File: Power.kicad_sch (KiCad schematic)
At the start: 19 parts, among them U2 sct2620

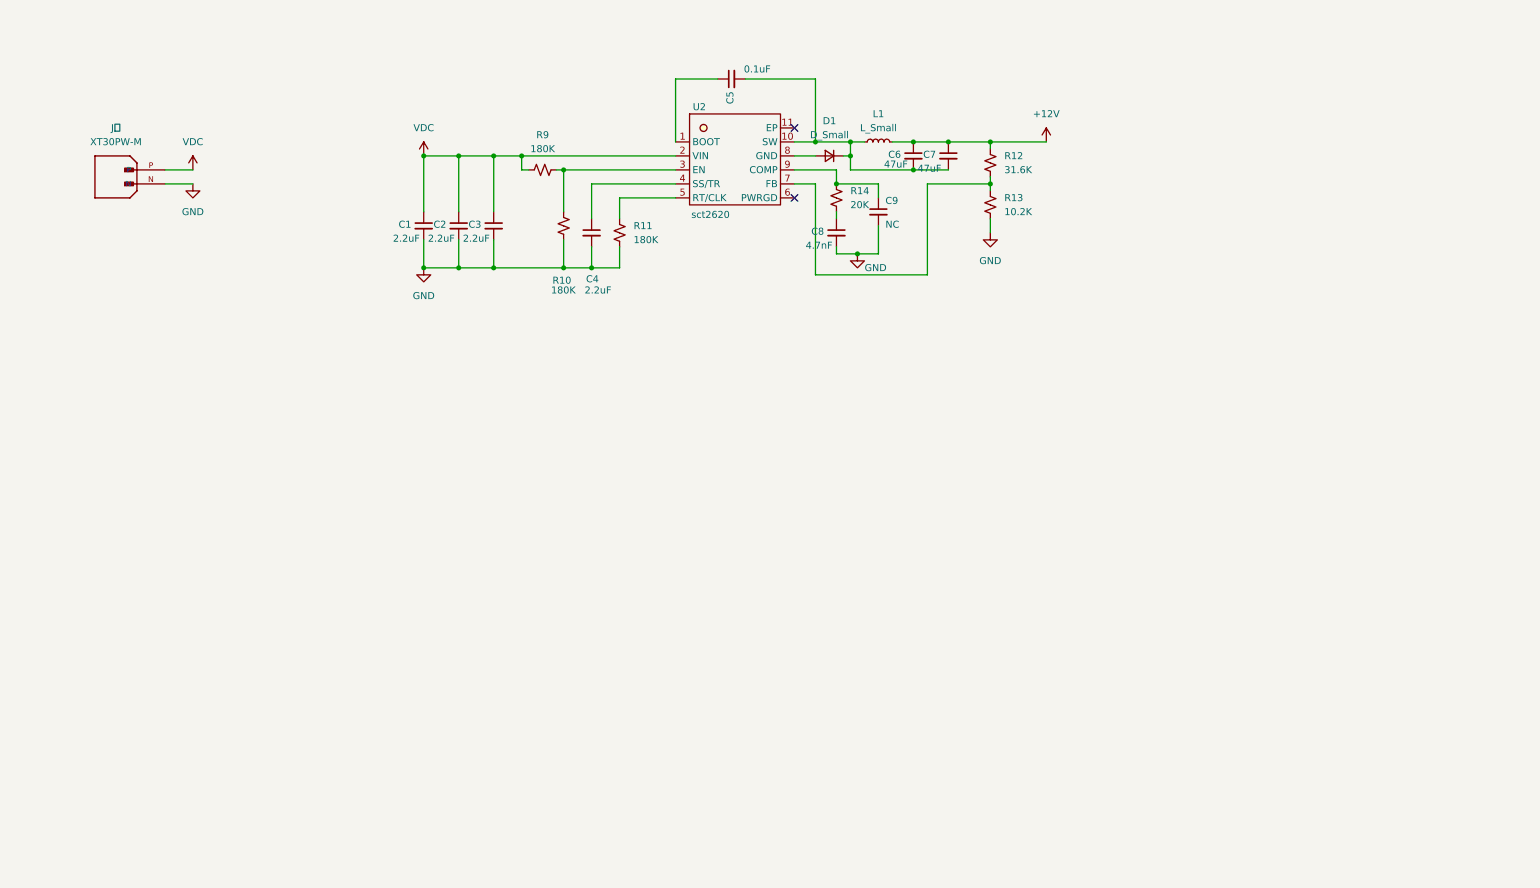
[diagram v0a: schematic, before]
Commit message: 优化电源原理图设计
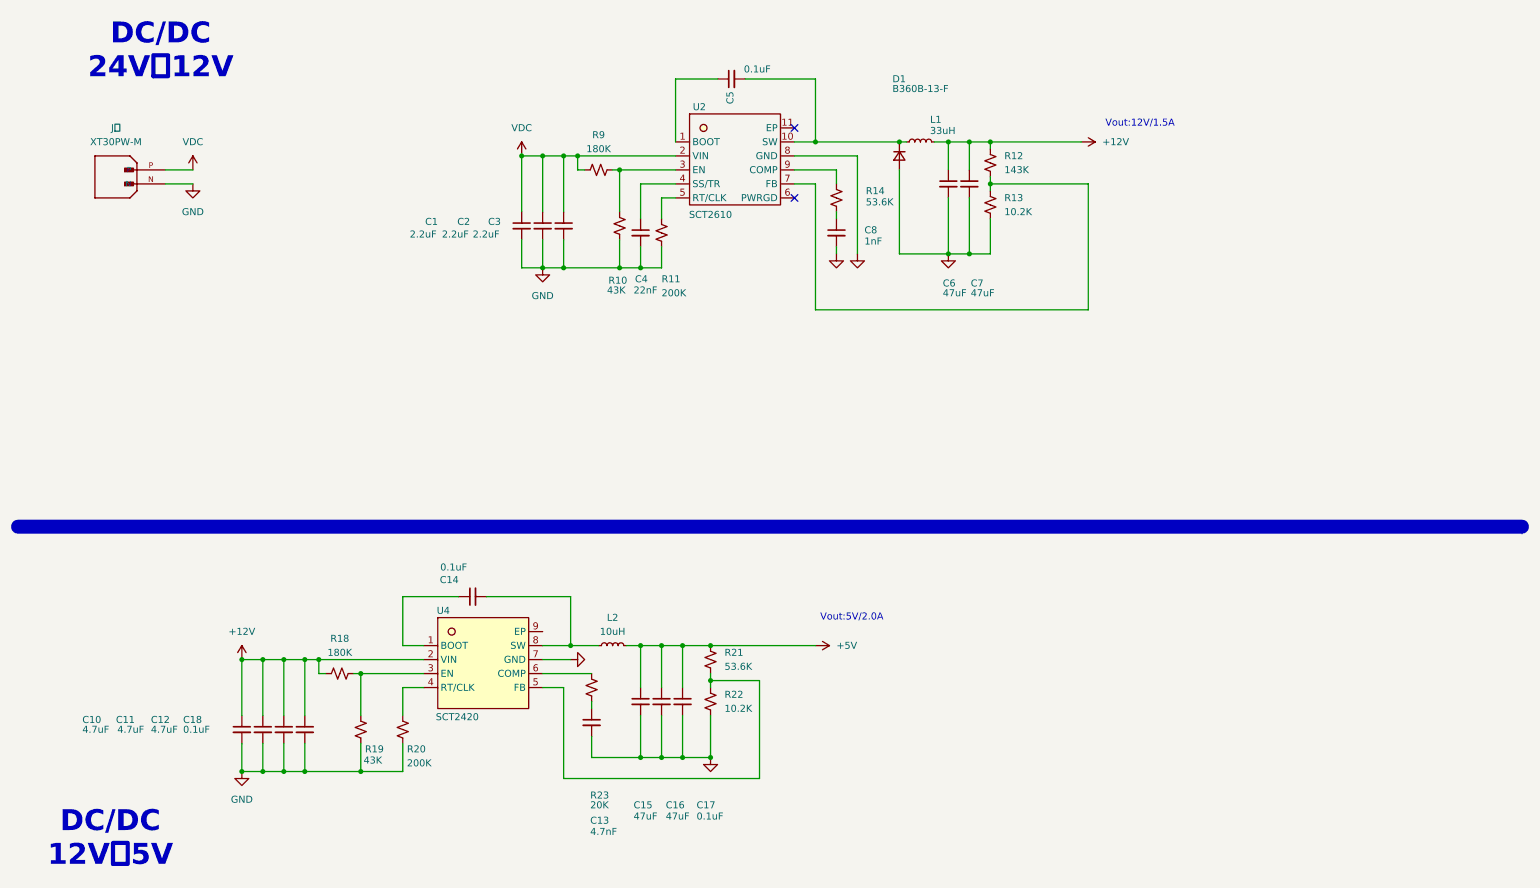
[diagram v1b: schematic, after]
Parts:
- removed C9: NC, symbol Device:C_Small
- added C10, C11, C12: 4.7uF, symbol Device:C_Small
- added C13: 4.7nF, symbol Device:C_Small
- added C14, C17, C18: 0.1uF, symbol Device:C_Small
- added C15, C16: 47uF, symbol Device:C_Small
- added L2: 10uH, symbol Device:L_Small
- added R18: 180K, symbol Device:R_Small_US
- added R19: 43K, symbol Device:R_Small_US
- added R20: 200K, symbol Device:R_Small_US
- added R21: 53.6K, symbol Device:R_Small_US
- added R22: 10.2K, symbol Device:R_Small_US
- added R23: 20K, symbol Device:R_Small_US
- added U4: SCT2420, Package_SO:SOIC-8_5.3x6.2mm_P1.27mm, symbol User_Driver:SCT2420
- C4: value 2.2uF -> 22nF
- C8: value 4.7nF -> 1nF
- D1: value D_Small -> B360B-13-F
- L1: value L_Small -> 33uH
- R10: value 180K -> 43K
- R11: value 180K -> 200K
- R12: value 31.6K -> 143K
- R14: value 20K -> 53.6K
- U2: value sct2620 -> SCT2610
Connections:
- net +12V: now also C10.1, C11.1, C12.1, C18.1, R18.1, U4.2 (VIN)
- net GND: now also C6.2, C7.2, D1.2 (A), U2.8 (GND), C10.2, C11.2, C12.2, C13.2, C15.2, C16.2, C17.2, C18.2, R19.1, R20.1, R22.2, U4.7 (GND)
- net at C5.2, D1.1 (K), L1.1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: no longer C6.2, C7.2
- new net: R18.2, R19.2, U4.3 (EN)
- new net: C13.1, R23.1
- new net: R23.2, U4.6 (COMP)
- new net: C14.1, U4.1 (BOOT)
- new net: C14.2, L2.1, U4.8 (SW)
- new net: R20.2, U4.4 (RT/CLK)
- new net: R21.2, R22.1, U4.5 (FB)
- new net +5V: C15.1, C16.1, C17.1, L2.2, R21.1
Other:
- note added: "DC/DC 12V转5V"
- note added: "DC/DC 24V转12V"
- note added: "Vout:12V/1.5A"
- note added: "Vout:5V/2.0A"
- moved on the sheet: C1, C2, C3, C4, C6, C7, D1, L1, R10, R11, R9
